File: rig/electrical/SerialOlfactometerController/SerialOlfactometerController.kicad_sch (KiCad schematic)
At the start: 34 parts, among them J1 Screw_Terminal_01x02, J10 Screw_Terminal_01x02, J11 Screw_Terminal_01x02, J12 Screw_Terminal_01x02, J13 Screw_Terminal_01x02, J14 Screw_Terminal_01x02, J15 Screw_Terminal_01x02, J16 Screw_Terminal_01x02, J17 Conn_01x05_Socket, J18 TST-105-01-X-D, J19 TST-105-01-X-D, J2 Screw_Terminal_01x02, J3 Screw_Terminal_01x02, J4 Screw_Terminal_01x02, J5 Screw_Terminal_01x02, J6 Screw_Terminal_01x02, J7 Screw_Terminal_01x02, J8 Screw_Terminal_01x02, J9 Screw_Terminal_01x02, U1 TPIC6595, U2 TPIC6595

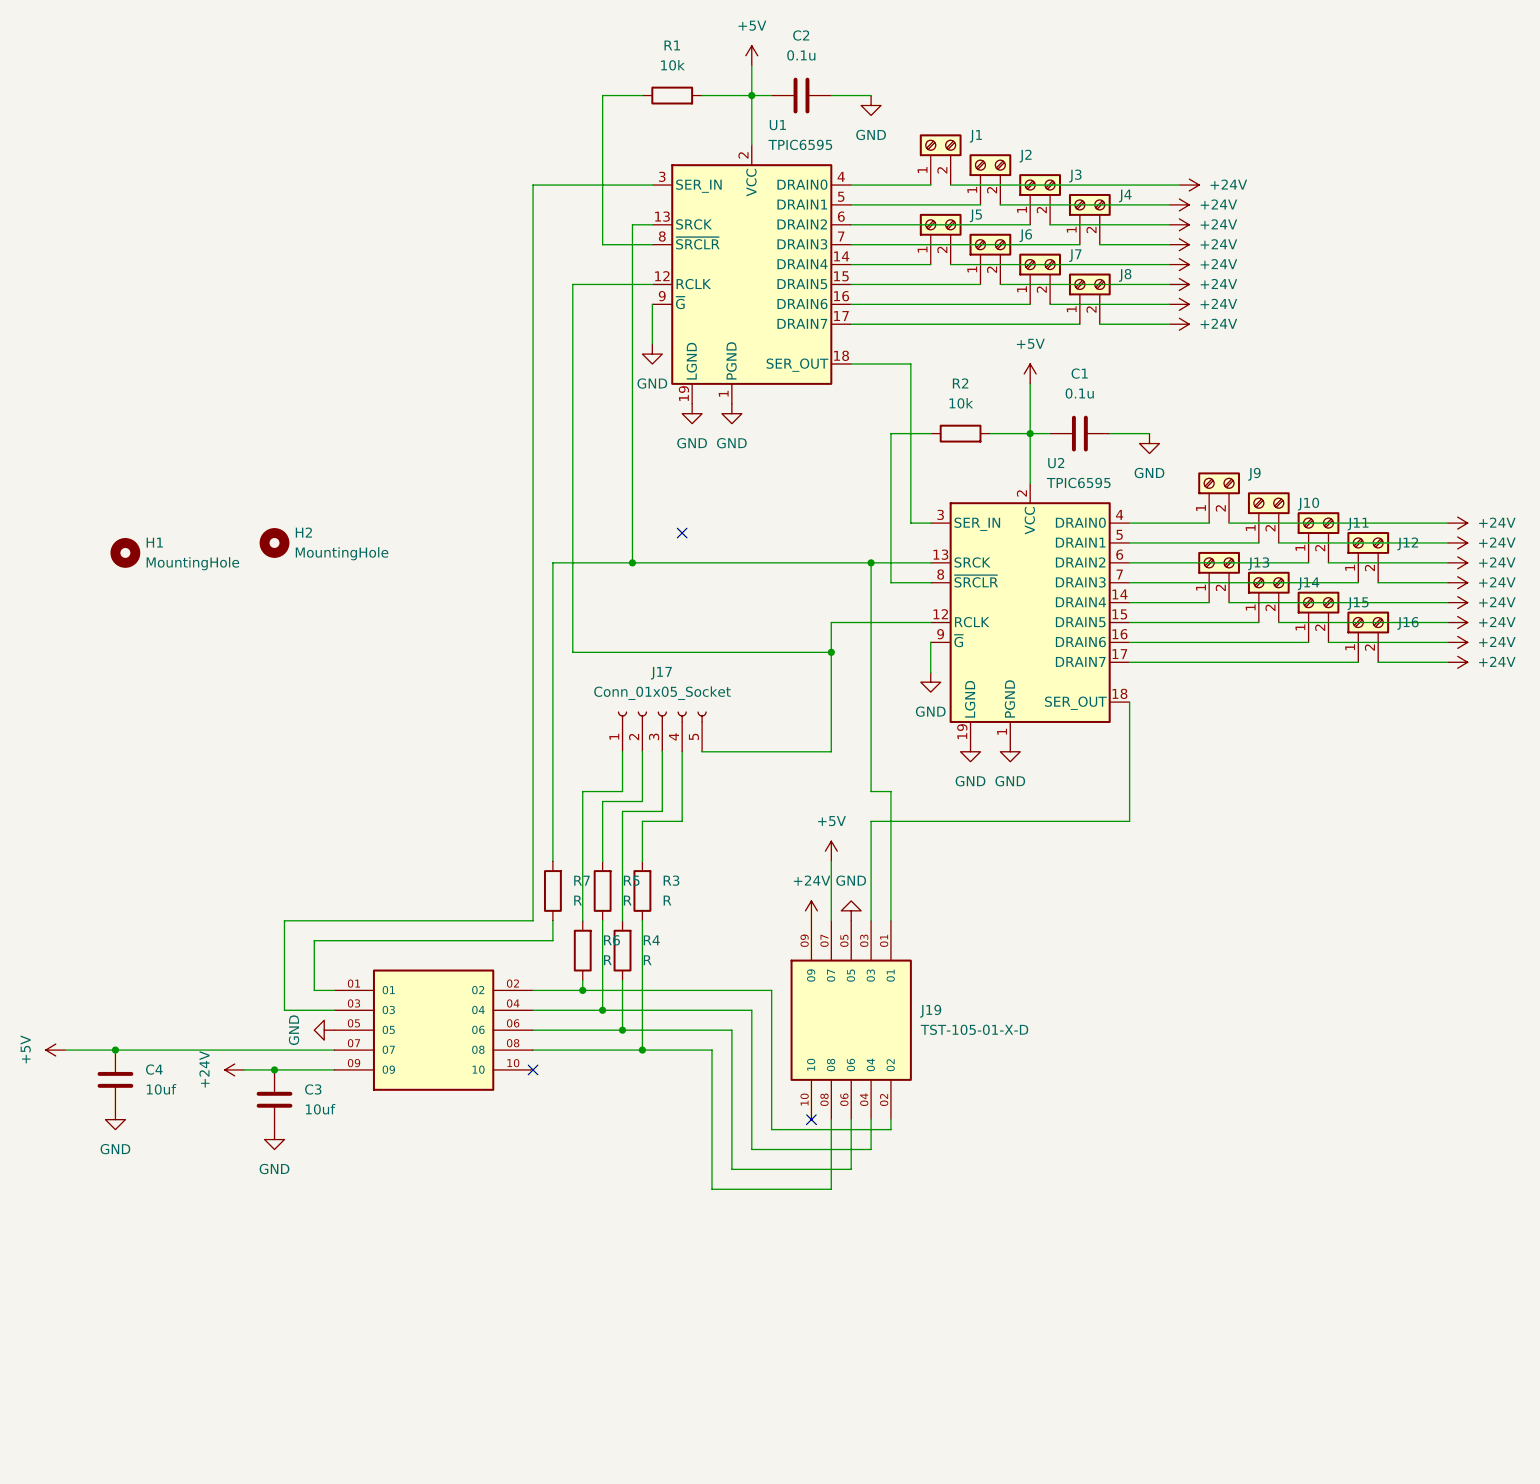
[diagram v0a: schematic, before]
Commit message: Serial Olfactometer improved design
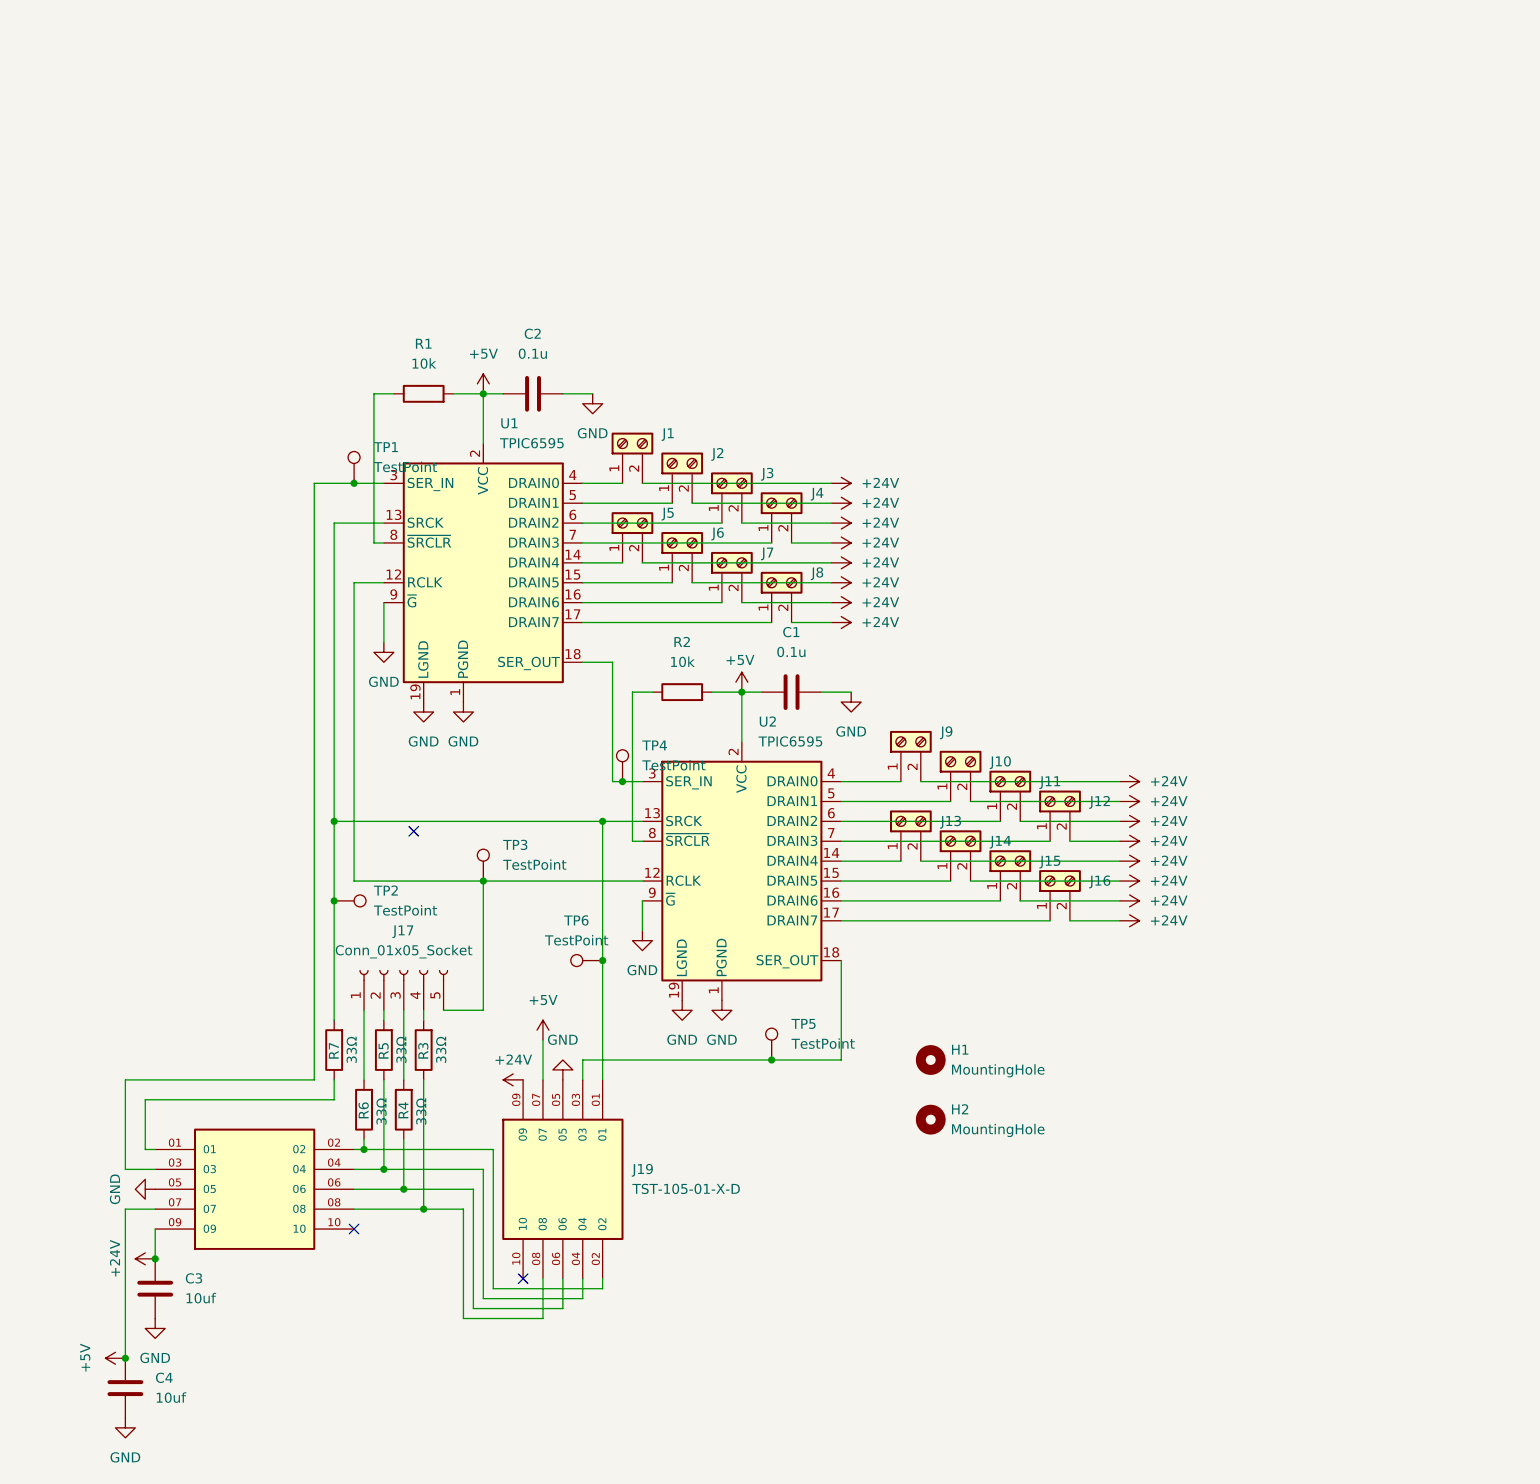
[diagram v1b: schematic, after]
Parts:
- added TP1, TP2, TP3, TP4, TP5, TP6: TestPoint, TestPoint:TestPoint_Pad_2.0x2.0mm, symbol Connector:TestPoint
- R3, R4, R5, R6, R7: value R -> 33Ω
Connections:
- net at J19.01, R7.2, U1.13 (SRCK)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: now also TP2.1, TP6.1
- net at J17.5 (Pin_5), U1.12 (RCLK), U2.12 (RCLK): now also TP3.1
- net at U1.18 (SER_OUT), U2.3 (SER_IN): now also TP4.1
- net at J18.03, U1.3 (SER_IN): now also TP1.1
- net at J19.03, U2.18 (SER_OUT): now also TP5.1
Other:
- company: (none) -> Ruta and Kronauer Labs, Rockefeller University
- title: (none) -> MultiBiOS Serial Olfactometer Controller
- moved on the sheet: C1, C2, C3, C4, H1, H2, J1, J10, J11, J12, J13, J14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
